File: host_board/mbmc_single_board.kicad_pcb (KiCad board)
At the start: 2 copper layers, 116.5 x 81.3 mm, 122 parts, among them IC1 ULN2803, IC15 PIC18F57K42-E_PT, IC16 REF3440IDBVR, IC17 MAX232, IC2 DIP Socket, IC3 REF02 5 VOLTS, IC4 5 VOLTS, IC5 12 VOLTS, IC6 3.3 VOLTS, J1 1-1586043-4, J2 1586044-4, Q3 ASF1, X15 RX-2, X16 TX-2, X17 RESETJMP

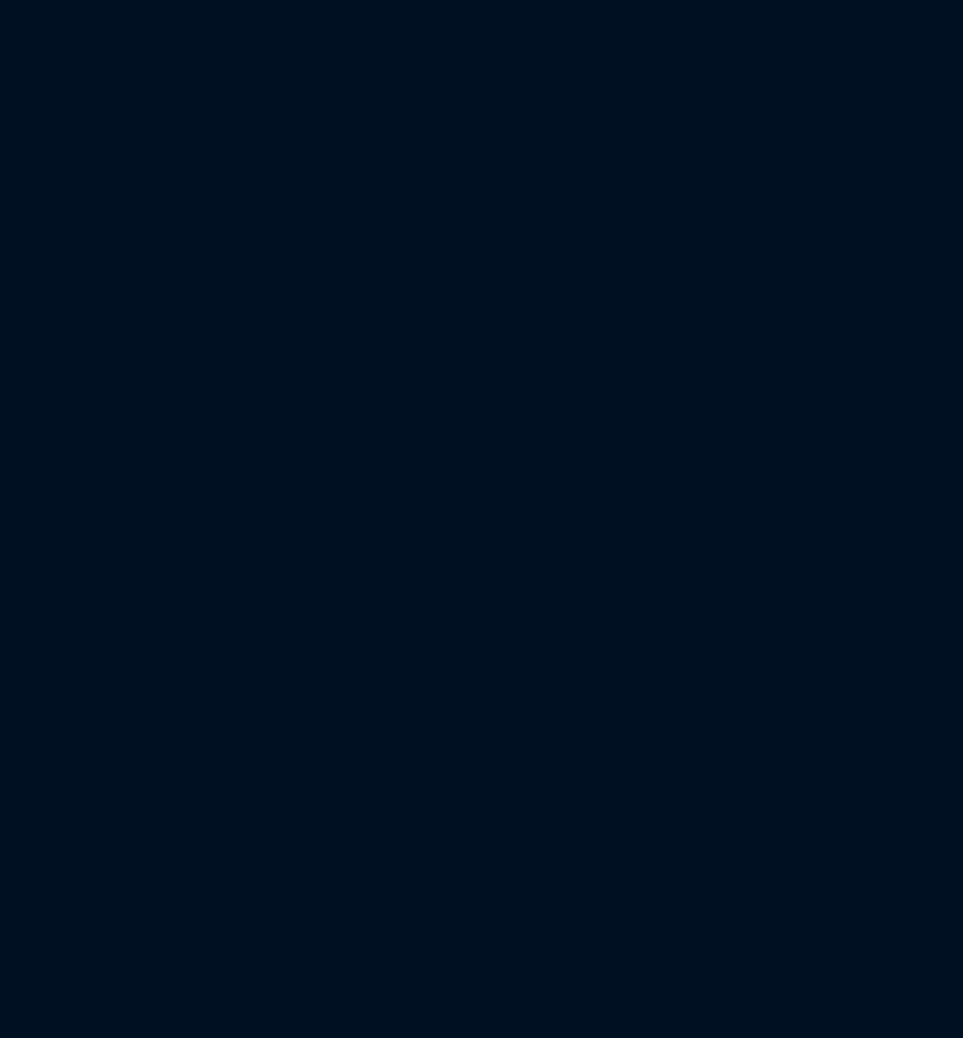
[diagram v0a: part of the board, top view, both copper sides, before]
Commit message: up
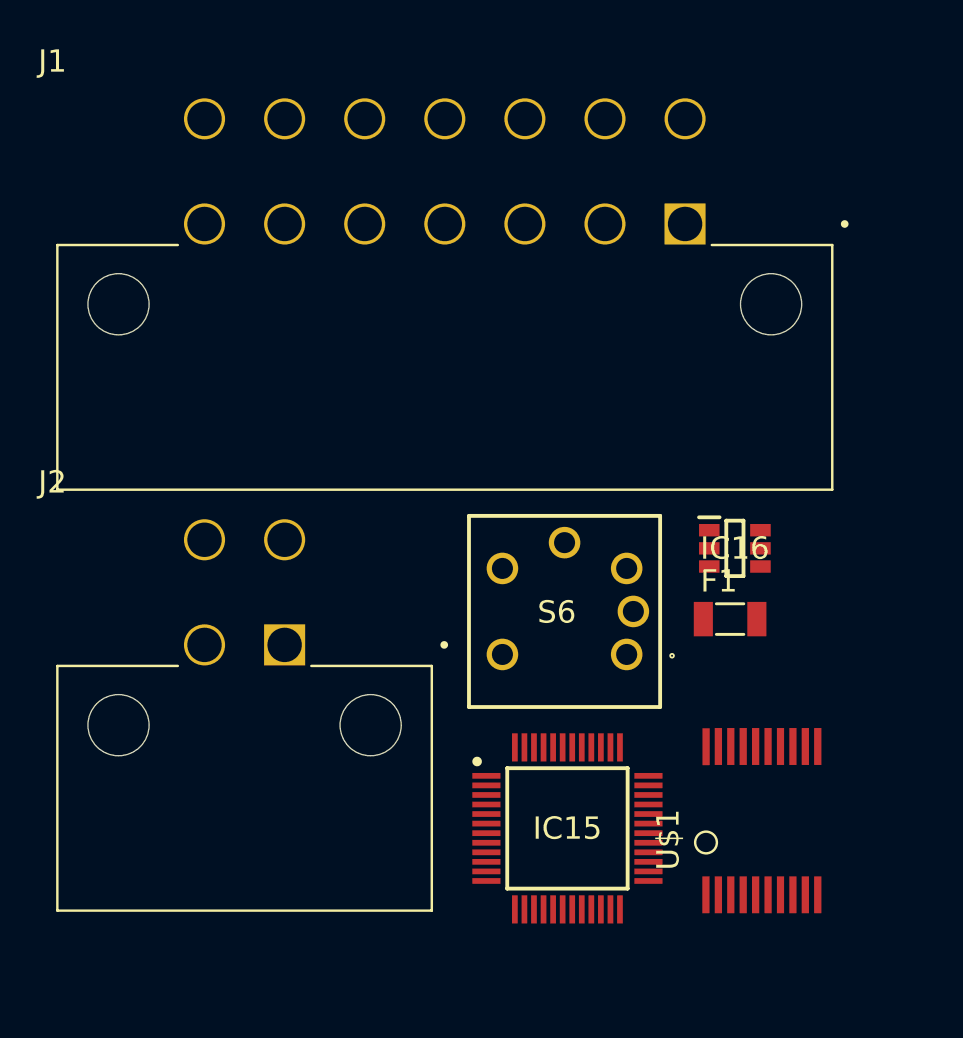
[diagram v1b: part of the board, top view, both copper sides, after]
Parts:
- added F1: ?1206L, mbmc_single_board:1206L, F.Cu at (35.5, 27.5)
- added IC15: PIC18F57K42-E_PT, mbmc_single_board:QFP50P900X900X120-48N, F.Cu at (27.0, 38.5)
- added IC16: REF3440IDBVR, mbmc_single_board:SOP95P280X145-6N, F.Cu at (35.7, 23.8)
- added J1: 1-1586043-4, mbmc_single_board:TE_1-1586043-4, F.Cu at (33.1, 6.85)
- added J2: 1586044-4, mbmc_single_board:TE_1586044-4, F.Cu at (12.2, 28.9)
- added S6: RESET SW, mbmc_single_board:B3W-9_1-LED, F.Cu at (26.8, 27.1)
- added U$1: MAX6818, mbmc_single_board:SSOP20, F.Cu at (37.1, 38.1)
- F1: value 1206L050 -> ?1206L
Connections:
- net CALIB_B renamed /CALIB_B
- net ENTER_B renamed /ENTER_B
- net EXT_INT1 renamed /EXT_INT1
- net SELECT_B renamed /SELECT_B
- F1 pad 1: ULN2803_24VDC -> /ULN2803_24VDC
- IC15 pad 1: N$245 -> Net-(IC15-RC7)
- IC15 pad 10: V_BBAT -> /V_BBAT
- IC15 pad 11: C_MPPT -> /C_MPPT
- IC15 pad 12: I5_ULN2803 -> /I5_ULN2803
- IC15 pad 13: MAX_EN1 -> /MAX_EN1
- IC15 pad 14: (no net) -> unconnected-(IC15-RF6-Pad14)
- IC15 pad 15: (no net) -> unconnected-(IC15-RF7-Pad15)
- IC15 pad 16: V_INVER -> /V_INVER
- IC15 pad 17: V_LIGHT_SEN -> /V_LIGHT_SEN
- IC15 pad 18: N$233 -> Net-(IC15-ICSPCLK/RB6)
- IC15 pad 19: N$232 -> Net-(IC15-ICSPDAT/RB7)
- IC15 pad 2: RELAYL1 -> /RELAYL1
- IC15 pad 20: N$231 -> Net-(IC15-VPP/~{MCLR}/RE3)
- IC15 pad 21: C_BATT -> /C_BATT
- IC15 pad 22: C_PV -> /C_PV
- IC15 pad 23: V_CC -> /V_CC
- IC15 pad 24: VREF4.1 -> /VREF4.1
- IC15 pad 25: V_BAT -> /V_BAT
- IC15 pad 26: V_PV -> /V_PV
- IC15 pad 27: N$250 -> Net-(IC15-RE0)
- IC15 pad 28: N$251 -> Net-(IC15-RE1)
- IC15 pad 29: DLED -> /DLED
- IC15 pad 3: RELAYL2 -> /RELAYL2
- IC15 pad 30: N$22 -> Net-(IC15-VDD_1)
- IC15 pad 32: CLK16MHZCPU -> /CLK16MHZCPU
- IC15 pad 33: V_CMODE -> /V_CMODE
- IC15 pad 34: N$261 -> Net-(IC15-RC0)
- IC15 pad 35: N$259 -> Net-(IC15-RC1)
- IC15 pad 36: DAQ_CS0 -> /DAQ_CS0
- IC15 pad 37: IO_RF1 -> /IO_RF1
- IC15 pad 4: AC_CHARGER -> /AC_CHARGER
- IC15 pad 40: N$260 -> Net-(IC15-RC2)
- IC15 pad 41: N$258 -> Net-(IC15-RC3)
- IC15 pad 42: N$255 -> Net-(IC15-RD0)
- IC15 pad 43: PWM8 -> /PWM8
- IC15 pad 44: SW0 -> /SW0
- IC15 pad 46: N$67 -> Net-(IC15-RC4)
- IC15 pad 47: N$257 -> Net-(IC15-RC5)
- IC15 pad 48: N$247 -> Net-(IC15-RC6)
- IC15 pad 5: OUTP_3 -> /OUTP_3
- IC15 pad 7: N$22 -> Net-(IC15-VDD_1)
- IC15 pad 8: EXT_INT0 -> /EXT_INT0
- IC16 pad 5: VREF4.1 -> /VREF4.1
- IC16 pad 6: VREF4.1 -> /VREF4.1
- J1 pad 1: ANA0_IN_C_BAT -> /ANA0_IN_C_BAT
- J1 pad 10: ANB5_IN_V_L_SENSOR -> /ANB5_IN_V_L_SENSOR
- J1 pad 14: VREF5V -> /VREF5V
- J1 pad 2: ANA1_IN_C-PV -> /ANA1_IN_C-PV
- J1 pad 3: ANA2_IN_V_CC -> /ANA2_IN_V_CC
- J1 pad 4: ANA4_IN_V_BAT -> /ANA4_IN_V_BAT
- J1 pad 5: ANA5_IN_V_PV -> /ANA5_IN_V_PV
- J1 pad 6: ANA6_IN_V_CMODE -> /ANA6_IN_V_CMODE
- J1 pad 7: ANB2_IN_V_BBAT -> /ANB2_IN_V_BBAT
- J1 pad 8: ANB3_IN_C_MPPT -> /ANB3_IN_C_MPPT
- J1 pad 9: ANB4_IN_V_INVERTER -> /ANB4_IN_V_INVERTER
- S6 pad 1: (no net) -> unconnected-(S6-Pad1)
- S6 pad 3: (no net) -> unconnected-(S6-Pad3)
- S6 pad 4: N$299 -> Net-(X17B-S)
- S6 pad 5: N$249 -> Net-(S6-+)
- U$1 pad EN_L: MAX_EN1 -> /MAX_EN1
- U$1 pad IN1: N$44 -> Net-(INP0B-S)
- U$1 pad IN2: N$46 -> Net-(INP0A-S)
- U$1 pad IN3: N$47 -> Net-(INP0C-S)
- U$1 pad IN4: N$48 -> Net-(INP0D-S)
- U$1 pad IN5: N$49 -> Net-(INP0E-S)
- U$1 pad IN6: N$50 -> Net-(INP0F-S)
- U$1 pad IN7: N$51 -> Net-(INP0G-S)
- U$1 pad IN8: N$52 -> Net-(INP0H-S)
- U$1 pad OUT1: DAQ_CS0 -> /DAQ_CS0
- U$1 pad OUT2: IO_RF1 -> /IO_RF1
- U$1 pad OUT6: SW0 -> /SW0
- U$1 pad OUT7: SL3_PIN3 -> /SL3_PIN3
- U$1 pad OUT8: DEBUG8_LED -> /DEBUG8_LED
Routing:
- net V_PV: vias 1 -> 0
- net V_LIGHT_SEN: vias 7 -> 0
- net V_INVER: vias 4 -> 0
- net V_CMODE: vias 2 -> 0
- net V_CC: vias 4 -> 0
- net V_BBAT: vias 2 -> 0
- net V_BAT: vias 7 -> 0
- net VREF4.1: vias 5 -> 0
- net SW0: vias 6 -> 0
- net SL3_PIN3: vias 2 -> 0
- net RELAYL2: vias 3 -> 0
- net RELAYL1: vias 4 -> 0
- net PWM8: vias 4 -> 0
- net OUTP_3: vias 5 -> 0
- net Net-(X17B-S): vias 0 -> 4
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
